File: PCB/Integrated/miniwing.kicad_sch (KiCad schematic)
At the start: 69 parts, among them U1 rp2040-zero

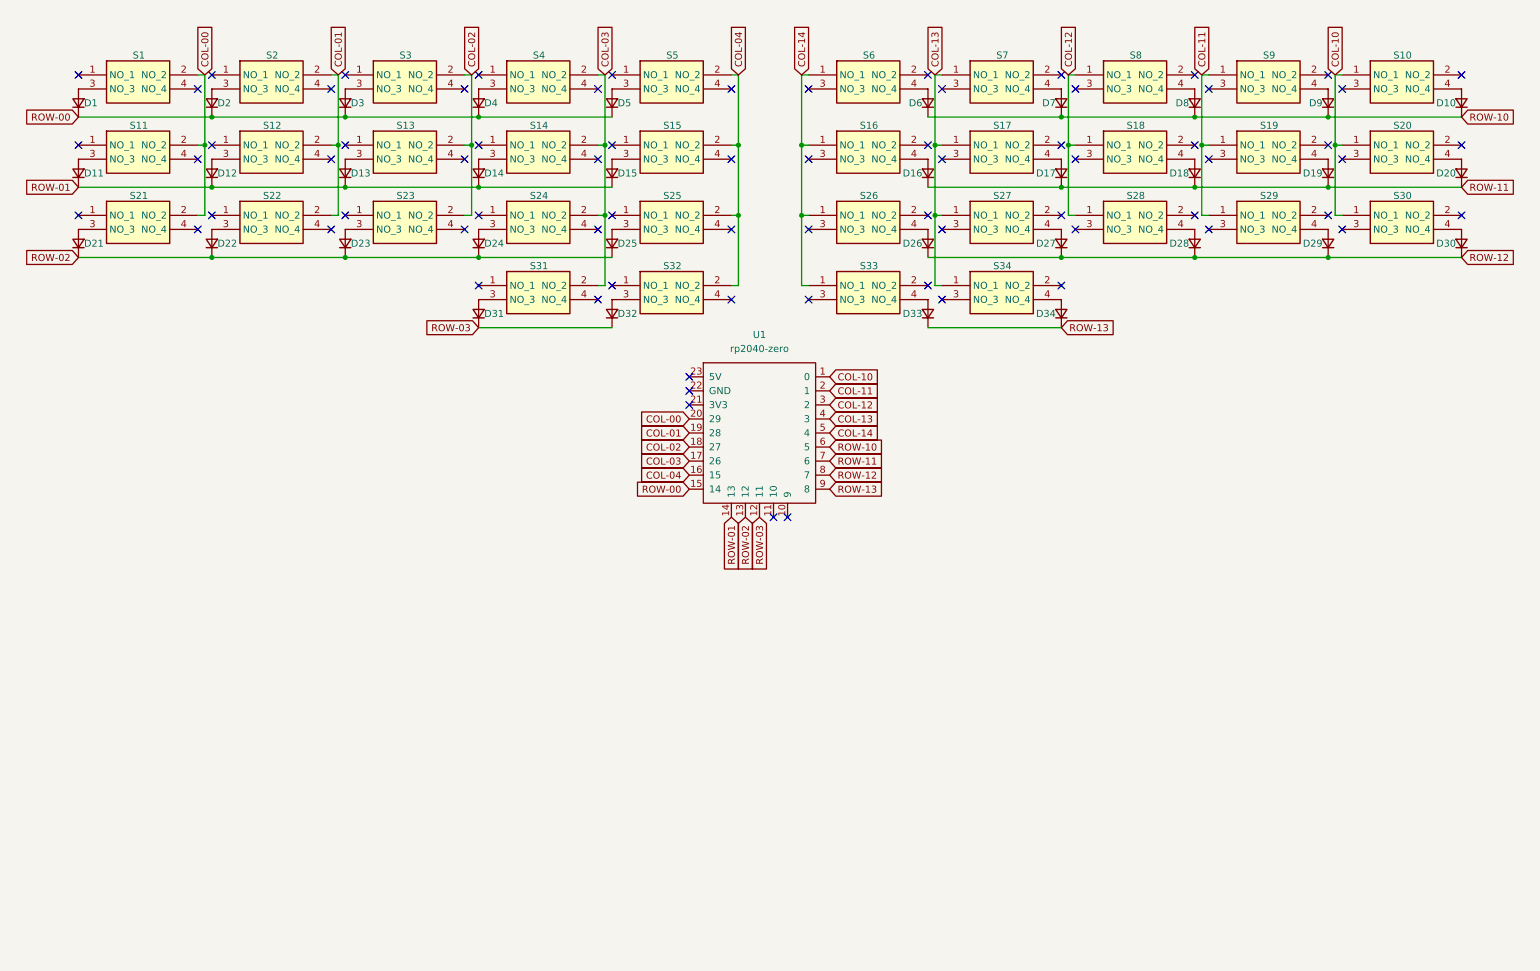
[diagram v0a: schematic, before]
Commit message: Hopefully complete first version of integrated pcb.
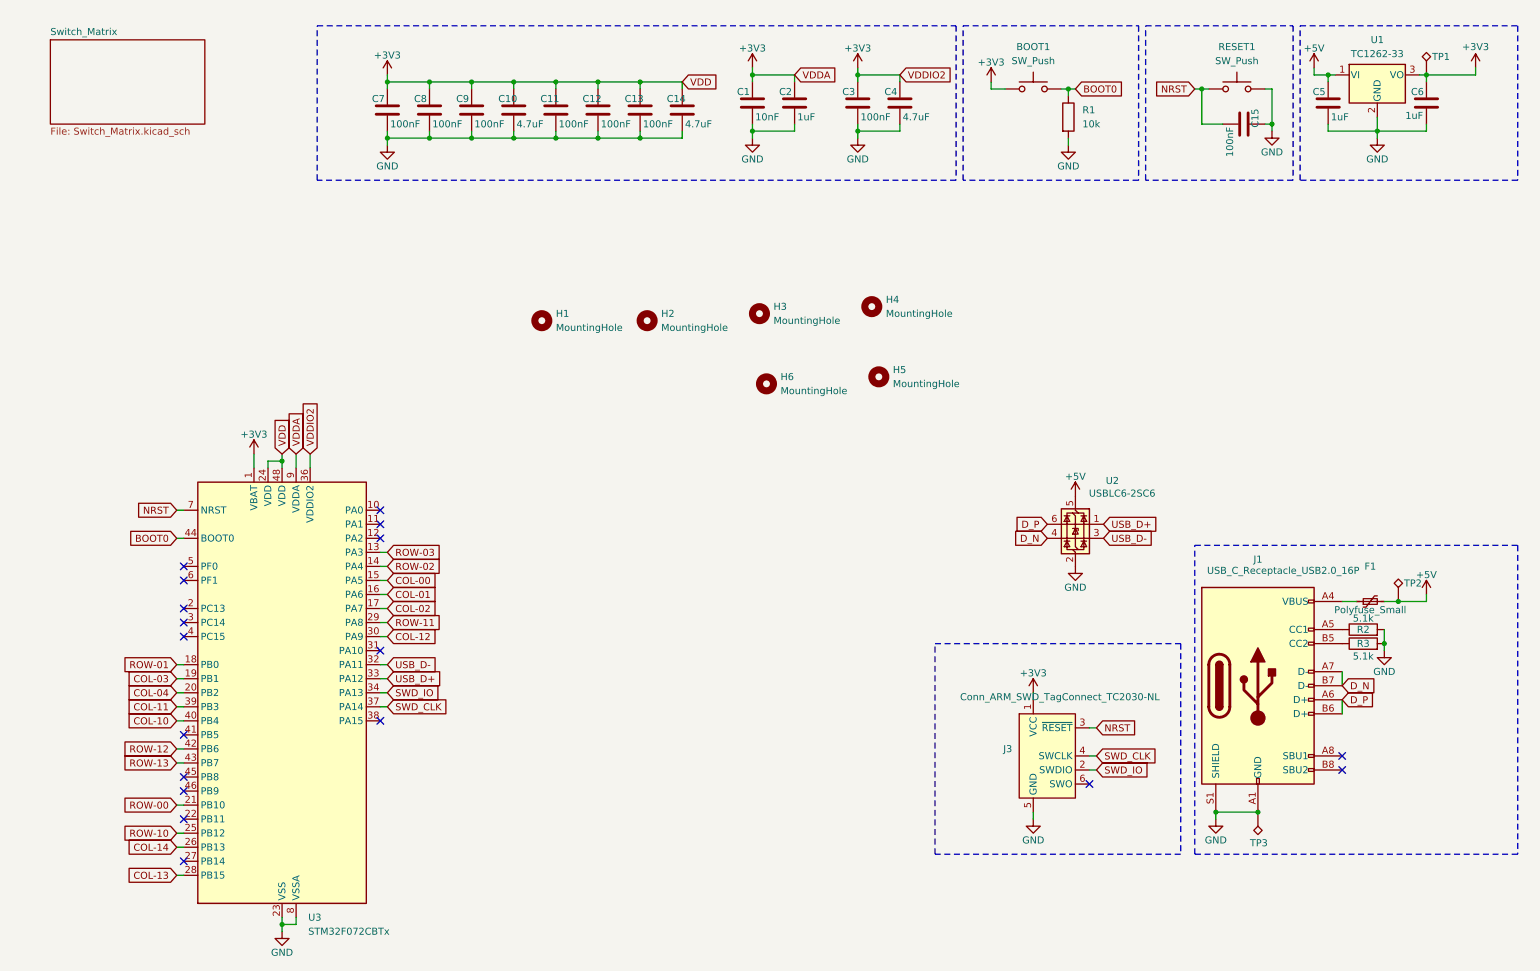
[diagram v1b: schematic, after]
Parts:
- removed D1, D10, D11, D12, D13, D14, D15, D16, D17, D18, D19, D2, D20, D21, D22, D23, D24, D25, D26, D27, D28, D29, D3, D30, D31, D32, D33, D34, D4, D5, D6, D7, D8, D9: D_Small, Diode_SMD:D_SOD-123, symbol Device:D_Small
- removed S1, S10, S11, S12, S13, S14, S15, S16, S17, S18, S19, S2, S20, S21, S22, S23, S24, S25, S26, S27, S28, S29, S3, S30, S31, S32, S33, S34, S4, S5, S6, S7, S8, S9: SKHCBKA010, KiCad:SKHCBKA010, symbol SKHCBKA010:SKHCBKA010
- removed U1: rp2040-zero, mcu:rp2040-zero-tht, symbol mcu:rp2040-zero
- added BOOT1, RESET1: SW_Push, Button_Switch_SMD:SW_Push_1P1T_XKB_TS-1187A, symbol Switch:SW_Push
- added C1: 10nF, Capacitor_SMD:C_0402_1005Metric, symbol Device:C
- added C10, C14, C4: 4.7uF, Capacitor_SMD:C_0402_1005Metric, symbol Device:C
- added C11, C12, C13, C15, C3, C7, C8, C9: 100nF, Capacitor_SMD:C_0402_1005Metric, symbol Device:C
- added C2, C5, C6: 1uF, Capacitor_SMD:C_0402_1005Metric, symbol Device:C
- added F1: Polyfuse_Small, Fuse:Fuse_1812_4532Metric, symbol Device:Polyfuse_Small
- added H1, H2, H3, H4, H5, H6: MountingHole, MountingHole:MountingHole_3.2mm_M3, symbol Mechanical:MountingHole
- added J1: USB_C_Receptacle_USB2.0_16P, Connector_USB:USB_C_Receptacle_HRO_TYPE-C-31-M-12, symbol Connector:USB_C_Receptacle_USB2.0_16P
- added J3: Conn_ARM_SWD_TagConnect_TC2030-NL, Connector:Tag-Connect_TC2030-IDC-NL_2x03_P1.27mm_Vertical, symbol Connector:Conn_ARM_SWD_TagConnect_TC2030-NL
- added R1: 10k, Resistor_SMD:R_0603_1608Metric, symbol Device:R
- added R2, R3: 5.1k, Resistor_SMD:R_0603_1608Metric, symbol Device:R
- added TP1, TP2, TP3: TestPoint_Alt, TestPoint:TestPoint_Pad_1.0x1.0mm, symbol Connector:TestPoint_Alt
- added U1: TC1262-33, Package_TO_SOT_SMD:SOT-223-3_TabPin2, symbol Regulator_Linear:TC1262-33
- added U2: USBLC6-2SC6, Package_TO_SOT_SMD:SOT-23-6, symbol Power_Protection:USBLC6-2SC6
- added U3: STM32F072CBTx, Package_QFP:LQFP-48_7x7mm_P0.5mm, symbol MCU_ST_STM32F0:STM32F072CBTx
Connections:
- net COL-00: now also U3.15 (PA5)
- net COL-01: now also U3.16 (PA6)
- net COL-02: now also U3.17 (PA7)
- net COL-03: now also U3.19 (PB1)
- net COL-04: now also U3.20 (PB2)
- net COL-10: now also U3.40 (PB4)
- net COL-11: now also U3.39 (PB3)
- net COL-12: now also U3.30 (PA9)
- net COL-13: now also U3.28 (PB15)
- net COL-14: now also U3.26 (PB13)
- net ROW-00: now also U3.21 (PB10)
- net ROW-01: now also U3.18 (PB0)
- net ROW-02: now also U3.14 (PA4)
- net ROW-03: now also U3.13 (PA3)
- net ROW-10: now also U3.25 (PB12)
- net ROW-11: now also U3.29 (PA8)
- net ROW-12: now also U3.42 (PB6)
- net ROW-13: now also U3.43 (PB7)
- new net: F1.1, J1.A4 (VBUS), J1.A9 (VBUS), J1.B4 (VBUS), J1.B9 (VBUS)
- new net: J1.B5 (CC2), R3.1
- new net: J1.A5 (CC1), R2.1
- new net +3V3: BOOT1.1, C1.1, C10.1, C11.1, C12.1, C13.1, C14.1, C2.1, C3.1, C4.1, C6.1, C7.1, C8.1, C9.1, J3.1 (VCC), TP1.1, U1.3 (VO), U3.1 (VBAT), U3.24 (VDD), U3.36 (VDDIO2), U3.48 (VDD), U3.9 (VDDA)
- new net +5V: C5.1, F1.2, TP2.1, U1.1 (VI), U2.5 (VBUS)
- new net BOOT0: BOOT1.2, R1.1, U3.44 (BOOT0)
- new net D_N: J1.A7 (D-), J1.B7 (D-), U2.4 (I/O2)
- new net D_P: J1.A6 (D+), J1.B6 (D+), U2.6 (I/O1)
- new net GND: C1.2, C10.2, C11.2, C12.2, C13.2, C14.2, C15.1, C2.2, C3.2, C4.2, C5.2, C6.2, C7.2, C8.2, C9.2, J1.A1 (GND), J1.A12 (GND), J1.B1 (GND), J1.B12 (GND), J1.S1 (SHIELD), J3.5 (GND), R1.2, R2.2, R3.2, RESET1.2, TP3.1, U1.2 (GND), U2.2 (GND), U3.23 (VSS), U3.35 (VSS), U3.47 (VSS), U3.8 (VSSA)
- new net NRST: C15.2, J3.3 (~{RESET}), RESET1.1, U3.7 (NRST)
- new net SWD_CLK: J3.4 (SWCLK), U3.37 (PA14)
- new net SWD_IO: J3.2 (SWDIO), U3.34 (PA13)
- new net USB_D+: U2.1 (I/O1), U3.33 (PA12)
- new net USB_D-: U2.3 (I/O2), U3.32 (PA11)
- no-connect marks 73 -> 18
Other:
- added sheet Switch_Matrix (Switch_Matrix.kicad_sch)
